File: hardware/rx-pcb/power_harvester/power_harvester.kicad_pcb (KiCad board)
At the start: 4 copper layers, 59 x 58 mm, 36 parts, among them J1 Conn_Coaxial_Small, J2 Conn_01x02_Pin

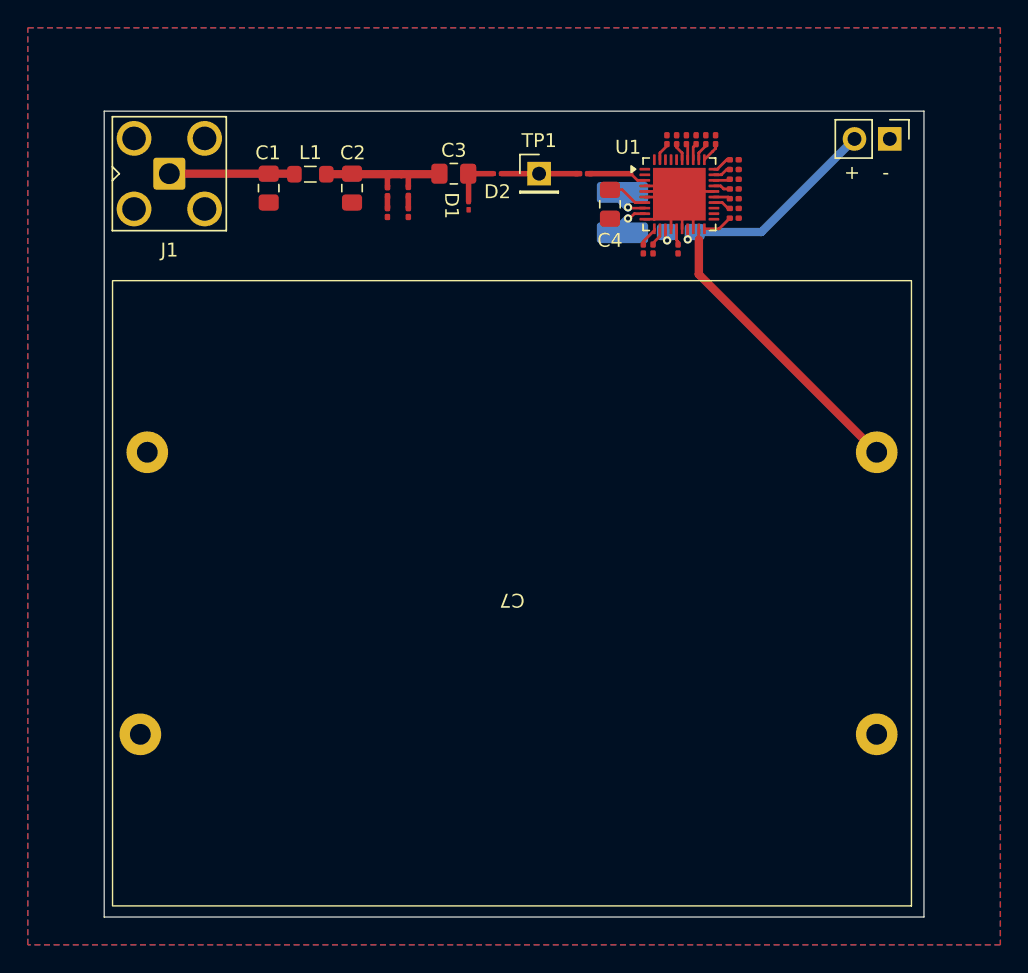
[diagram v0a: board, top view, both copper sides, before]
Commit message: power harvester updates and cleanup
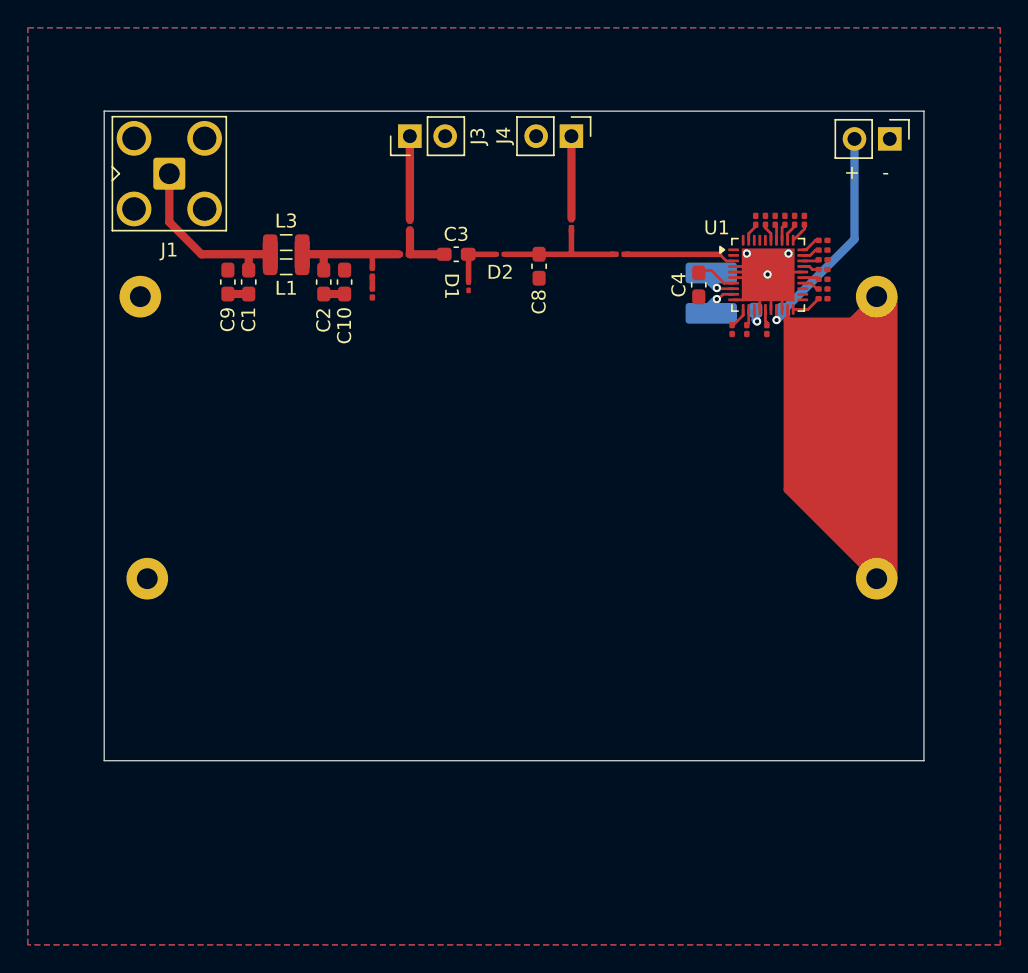
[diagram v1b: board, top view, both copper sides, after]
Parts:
- removed D5, D6: D_Zener, Capacitor_SMD:C_0201_0603Metric
- removed TP1: Conn_01x01_Pin, Connector_PinHeader_2.54mm:PinHeader_1x01_P2.54mm_Vertical
- added C10: C, Capacitor_SMD:C_0603_1608Metric_Pad1.08x0.95mm_HandSolder, F.Cu at (113.8, 87.3)
- added C8: 22u, Capacitor_SMD:C_0603_1608Metric_Pad1.08x0.95mm_HandSolder, F.Cu at (127.8, 86.2)
- added C9: C, Capacitor_SMD:C_0603_1608Metric_Pad1.08x0.95mm_HandSolder, F.Cu at (105.4, 87.3)
- added J3: Conn_Coaxial_Small, Connector_PinHeader_2.54mm:PinHeader_1x02_P2.54mm_Vertical, F.Cu at (118.5, 76.8)
- added J4: Conn_Coaxial_Small, Connector_PinHeader_2.54mm:PinHeader_1x02_P2.54mm_Vertical, F.Cu at (130.1, 76.8)
- added L3: L, Inductor_SMD:L_0805_2012Metric_Pad1.05x1.20mm_HandSolder, F.Cu at (109.6, 84.5)
- added R18: 0, Resistor_SMD:R_0201_0603Metric_Pad0.64x0.40mm_HandSolder, F.Cu at (118.1, 85.3)
- added R19: 0, Resistor_SMD:R_0201_0603Metric_Pad0.64x0.40mm_HandSolder, F.Cu at (118.5, 83.2)
- added R20: 0, Resistor_SMD:R_0201_0603Metric_Pad0.64x0.40mm_HandSolder, F.Cu at (130.1, 83.1)
- C1, C2, C4, C5, C6: footprint Capacitor_SMD:C_0805_2012Metric_Pad1.18x1.45mm_HandSolder -> Capacitor_SMD:C_0603_1608Metric_Pad1.08x0.95mm_HandSolder
- C3: value C -> 1n; footprint Capacitor_SMD:C_0805_2012Metric_Pad1.18x1.45mm_HandSolder -> Capacitor_SMD:C_0603_1608Metric_Pad1.08x0.95mm_HandSolder
- C7: moved to B.Cu
- moved C7 11.2 mm to (125.8, 98.5)
- moved R6 8.90 mm to (142.8, 90.7)
- moved C5 8.63 mm to (143.4, 88.5)
- moved C6 8.63 mm to (145.4, 88.5)
- moved R3 8.63 mm to (148.2, 86.4)
- moved R1 8.63 mm to (148.2, 85.7)
- moved R10 8.63 mm to (146.9, 82.9)
- moved R11 8.63 mm to (148.2, 88.5)
- moved R12 8.63 mm to (145.5, 82.9)
- moved R14 8.63 mm to (148.2, 87.8)
- moved R15 8.63 mm to (148.2, 84.3)
- moved R2 8.63 mm to (144.1, 82.9)
- moved R4 8.63 mm to (148.2, 87.1)
- moved R8 8.63 mm to (143.4, 82.9)
- moved R9 8.63 mm to (148.2, 85.0)
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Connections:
- C1 pad 2: GND -> Net-(C1-Pad2)
- C2 pad 2: GND -> Net-(C10-Pad1)
- C3 pad 1: Net-(D3-K) -> Net-(C3-Pad1)
- L1 pad 1: Net-(J1-In) -> Net-(D3-K)
- L1 pad 2: Net-(D3-K) -> Net-(J1-In)
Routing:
- net /bank: track 21.4 -> 49.5 mm
- net Net-(J3-In): track 0.00 -> 5.99 mm
- net Net-(J4-In): track 0.00 -> 5.89 mm
- net Net-(D2-K): track 5.49 -> 9.69 mm
- net Net-(C3-Pad1): track 0.00 -> 3.90 mm
- net /Pin: track 4.20 -> 7.96 mm
- net Net-(J1-In): track 9.02 -> 12.8 mm
- net Net-(C10-Pad1): track 0.00 -> 1.50 mm
- net Net-(C1-Pad2): track 0.00 -> 1.50 mm
- net /Vint: track 0.69 -> 1.80 mm
- net Net-(D3-K): track 10.0 -> 9.04 mm
- net Net-(D5-A): track 0.88 -> 0.00 mm
- net /Po: track 15.8 -> 16.3 mm
- net GND: vias 0 -> 3
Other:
- board size 59 x 58 mm -> 59 x 46.8 mm
